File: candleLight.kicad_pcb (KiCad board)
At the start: 2 copper layers, 37.7 x 22.8 mm, 40 parts, among them P501 USB_OTG, U201 STM32F072C8Tx, U301 MCP1754ST-3302E/MB, U401 TJA1051/3, X501 CON_SWD, X502 SUB-D9, Y201 8MHz

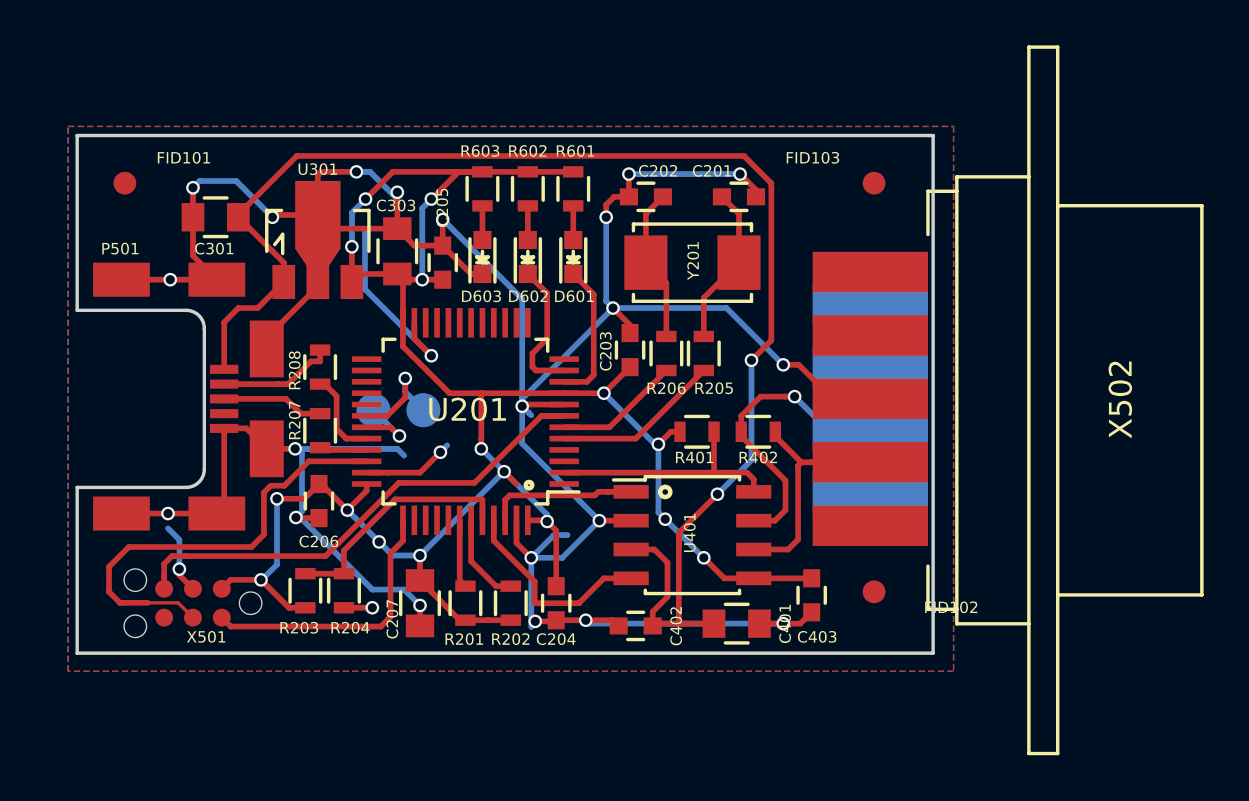
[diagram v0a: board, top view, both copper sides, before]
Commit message: candleLight v1.2
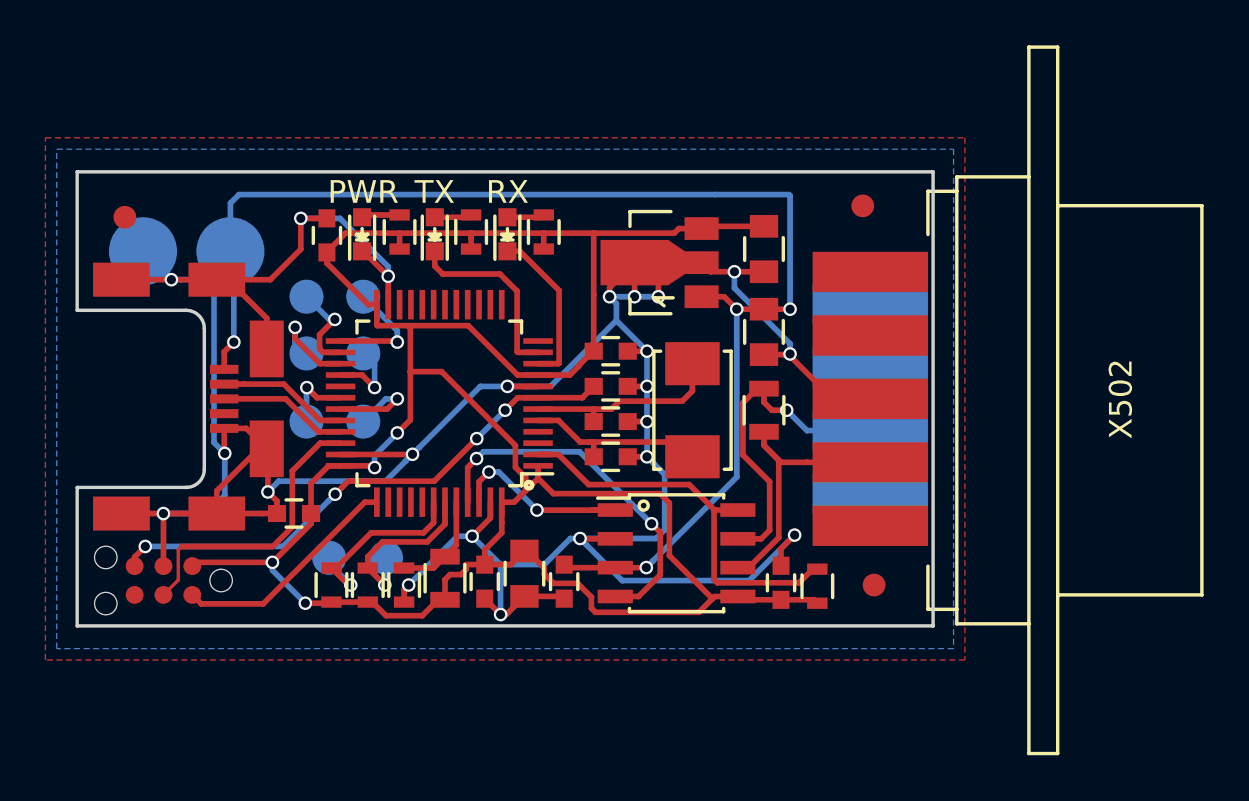
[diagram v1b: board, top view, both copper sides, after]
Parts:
- removed C401: 10uF, Capacitors_SMD:C_0805
- removed R205, R206: 0R, Resistors_SMD:R_0603
- removed R207, R208: 22R, Resistors_SMD:R_0603
- added C208: 100nF, Capacitors_SMD:C_0603, F.Cu at (64.9, 84.5)
- added CS: TEST_1P, Measurement_Points:Measurement_Point_Round-SMD-Pad_Small, B.Cu at (54.0, 80.5)
- added MISO: TEST_1P, Measurement_Points:Measurement_Point_Round-SMD-Pad_Small, B.Cu at (51.5, 83.0)
- added MOSI: TEST_1P, Measurement_Points:Measurement_Point_Round-SMD-Pad_Small, B.Cu at (54.0, 83.0)
- added SCK: TEST_1P, Measurement_Points:Measurement_Point_Round-SMD-Pad_Small, B.Cu at (51.5, 80.5)
- added SCL: TEST_1P, Measurement_Points:Measurement_Point_Round-SMD-Pad_Small, B.Cu at (52.5, 92.0)
- added SDA: TEST_1P, Measurement_Points:Measurement_Point_Round-SMD-Pad_Small, B.Cu at (55.0, 92.0)
- added W301: TEST_1P, Measurement_Points:Measurement_Point_Round-SMD-Pad_Big, B.Cu at (48.1, 78.5)
- added W302: TEST_1P, Measurement_Points:Measurement_Point_Round-SMD-Pad_Big, B.Cu at (44.3, 78.5)
- R203, R402: footprint Resistors_SMD:R_0603 -> Resistors_SMD:R_0805
- moved C301 24.7 mm to (71.7, 82.0), turned to 270 degrees
- moved C303 16.2 mm to (71.7, 78.4), turned to 270 degrees
- moved U301 15.1 mm to (67.0, 79.0), turned to 90 degrees
- moved C201 12.8 mm to (64.9, 87.5)
- moved C204 12.2 mm to (51.0, 90.0), turned to 180 degrees
- moved C202 10.0 mm to (64.9, 86.0), turned to 180 degrees
- moved R401 8.62 mm to (74.0, 93.2), turned to 90 degrees
- moved C206 8.12 mm to (59.4, 93.0)
- moved Y201 6.50 mm to (68.5, 85.5), turned to 90 degrees
- moved R202 6.35 mm to (54.2, 93.2)
- moved R203 6.17 mm to (57.6, 92.9)
- moved R201 5.95 mm to (52.6, 93.2)
- moved D603 5.39 mm to (54.0, 77.8)
- moved C205 5.24 mm to (52.4, 77.8)
- moved TX 5.17 mm to (51.5, 86.0)
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- renumbered W202 to RX, W201 to TX
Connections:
- FID101 pad ~: Net-(FID101-Pad~) -> (no net)
- FID102 pad ~: Net-(FID102-Pad~) -> (no net)
- FID103 pad ~: Net-(FID103-Pad~) -> (no net)
- P501 pad 4: Net-(P501-Pad4) -> (no net)
- R203 pad 2: Net-(R203-Pad2) -> /MCU/BOOT0
- R204 pad 1: Net-(R203-Pad2) -> GND
- R204 pad 2: GND -> /MCU/BOOT0
- U201 pad 12: Net-(U201-Pad12) -> (no net)
- U201 pad 13: Net-(U201-Pad13) -> (no net)
- U201 pad 14: Net-(U201-Pad14) -> (no net)
- U201 pad 15: Net-(U201-Pad15) -> (no net)
- U201 pad 16: Net-(U201-Pad16) -> (no net)
- U201 pad 17: Net-(U201-Pad17) -> (no net)
- U201 pad 18: Net-(U201-Pad18) -> (no net)
- U201 pad 19: Net-(U201-Pad19) -> (no net)
- U201 pad 20: Net-(U201-Pad20) -> (no net)
- U201 pad 21: Net-(U201-Pad21) -> (no net)
- U201 pad 22: Net-(U201-Pad22) -> (no net)
- U201 pad 29: Net-(U201-Pad29) -> (no net)
- U201 pad 3: Net-(U201-Pad3) -> (no net)
- U201 pad 32: Net-(R208-Pad2) -> /Connectors/USB_DM
- U201 pad 33: Net-(R207-Pad1) -> /Connectors/USB_DP
- U201 pad 38: Net-(U201-Pad38) -> (no net)
- U201 pad 39: Net-(U201-Pad39) -> (no net)
- U201 pad 4: Net-(U201-Pad4) -> (no net)
- U201 pad 40: Net-(U201-Pad40) -> (no net)
- U201 pad 41: Net-(U201-Pad41) -> (no net)
- U201 pad 44: Net-(R203-Pad2) -> /MCU/BOOT0
- U201 pad 5: Net-(R205-Pad2) -> Net-(C201-Pad2)
- U201 pad 6: Net-(R206-Pad1) -> Net-(C202-Pad2)
- X501 pad 6: Net-(X501-Pad6) -> (no net)
- X502 pad 1: Net-(X502-Pad1) -> (no net)
- X502 pad 4: Net-(X502-Pad4) -> (no net)
- X502 pad 5: Net-(X502-Pad5) -> (no net)
- X502 pad 6: Net-(X502-Pad6) -> (no net)
- X502 pad 8: Net-(X502-Pad8) -> (no net)
- X502 pad 9: Net-(X502-Pad9) -> (no net)
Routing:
- net +3V3: track 95.1 -> 115.2 mm, vias 16 -> 4
- net GND: track 166.1 -> 154.8 mm, vias 25 -> 22
- net Net-(R203-Pad2): track 10.9 -> 0.00 mm
- net Net-(R205-Pad2): track 7.39 -> 0.00 mm
- net /CAN/CAN_S: track 10.8 -> 18.2 mm
- net /MCU/CAN_RX: track 9.10 -> 16.0 mm, vias 0 -> 2
- net /Connectors/SWDIO: track 19.6 -> 12.8 mm
- net Net-(R201-Pad2): track 3.00 -> 8.98 mm, vias 0 -> 1
- net Net-(R206-Pad1): track 5.54 -> 0.00 mm
- net Net-(U201-Pad25): track 0.00 -> 5.14 mm, vias 0 -> 1
- net +5V: track 63.4 -> 58.4 mm, vias 2 -> 4
- net /MCU/BOOT0: track 0.00 -> 4.61 mm
- net Net-(U201-Pad27): track 0.00 -> 4.31 mm, vias 0 -> 1
- net Net-(U201-Pad26): track 0.00 -> 4.23 mm, vias 0 -> 1
- net Net-(R208-Pad2): track 3.89 -> 0.00 mm
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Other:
- board size 37.7 x 22.8 mm -> 37.7 x 20 mm
- board text added: "+5V"
- board text added: "CAN_H"
- board text added: "GND"
- board text added: "PWR"
- board text added: "RX"
- board text added: "TX"
- board text added: "candleLight v1.1"
- board text added: "http://bytewerk.org"
